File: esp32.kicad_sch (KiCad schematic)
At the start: 39 parts, among them U5 ESP32-S3R8, U6 W25Q128JVSIQ, Y1 40MHz

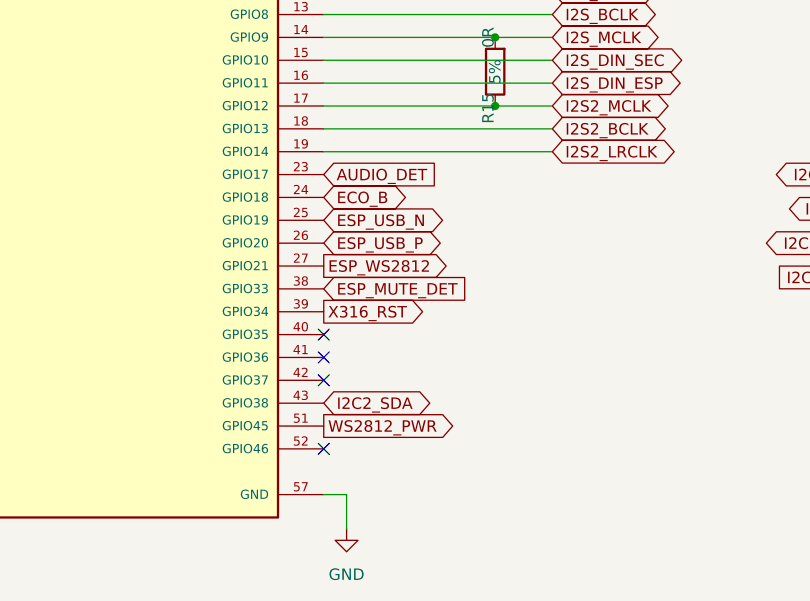
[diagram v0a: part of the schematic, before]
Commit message: rev2 update
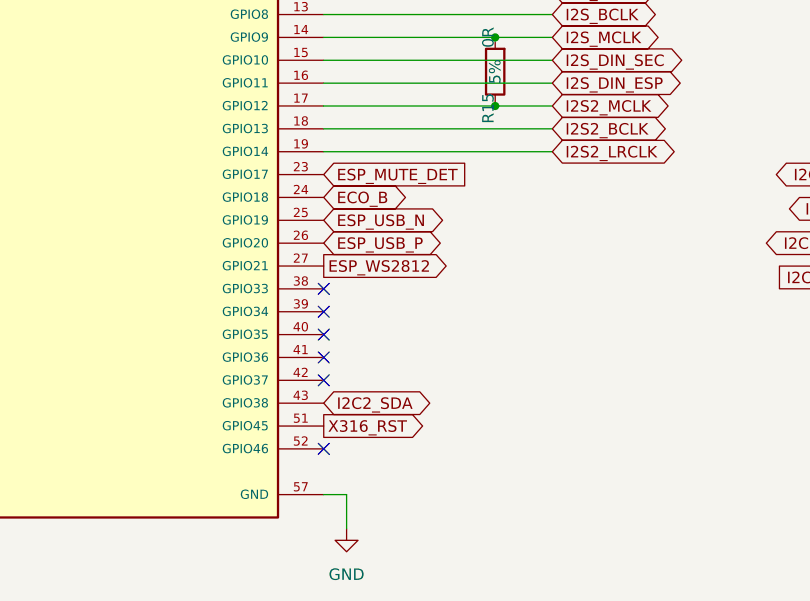
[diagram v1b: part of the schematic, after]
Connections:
- net AUDIO_DET is gone; now on net ESP_MUTE_DET: U5.23 (GPIO17)
- net WS2812_PWR is gone; now on net X316_RST: U5.51 (GPIO45)
- net ESP_MUTE_DET: no longer U5.38 (GPIO33)
- net X316_RST: no longer U5.39 (GPIO34)
- no-connect marks 6 -> 8
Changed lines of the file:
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@@
+	)
+	(no_connect
+		(at 162.56 116.84)
 	)
 	(no_connect
 		(at 162.56 134.62)
+	)
+	(no_connect
+		(at 162.56 119.38)
 	)
 	(no_connect
@@
 		)
 	)
+	(global_label "ESP_MUTE_DET"
+		(shape input)
+		(at 162.56 104.14 0)
+		(fields_autoplaced yes)
+		(effects
+			(font
+				(size 1.27 1.27)
+			)
+			(justify left)
+		)
+		(property "Intersheetrefs" "${INTERSHEET_REFS}"
+			(at 179.394 104.14 0)
+			(effects
+				(font
+					(size 1.27 1.27)
+				)
+				(justify left)
+				(hide yes)
+			)
+		)
+	)
 	(global_label "ESP_RX0"
 		(shape input)
@@
 		)
 	)
-	(global_label "X316_RST"
-		(shape output)
-		(at 162.56 119.38 0)
-		(fields_autoplaced yes)
-		(effects
-			(font
-				(size 1.27 1.27)
-			)
-			(justify left)
-		)
-		(property "Intersheetrefs" "${INTERSHEET_REFS}"
-			(at 174.7979 119.38 0)
-			(effects
-				(font
-					(size 1.27 1.27)
-				)
-				(justify left)
-				(hide yes)
-			)
-		)
-	)
 	(global_label "I2C_SCL"
 		(shape output)
@@
 		)
 	)
-	(global_label "ESP_MUTE_DET"
-		(shape input)
-		(at 162.56 116.84 0)
-		(fields_autoplaced yes)
-		(effects
-			(font
-				(size 1.27 1.27)
-			)
-			(justify left)
-		)
-		(property "Intersheetrefs" "${INTERSHEET_REFS}"
-			(at 179.394 116.84 0)
-			(effects
-				(font
-					(size 1.27 1.27)
-				)
-				(justify left)
-				(hide yes)
-			)
-		)
-	)
 	(global_label "ECO_B"
 		(shape bidirectional)
@@
 		)
 	)
+	(global_label "X316_RST"
+		(shape output)
+		(at 162.56 132.08 0)
+		(fields_autoplaced yes)
+		(effects
+			(font
+				(size 1.27 1.27)
+			)
+			(justify left)
+		)
+		(property "Intersheetrefs" "${INTERSHEET_REFS}"
+			(at 174.7979 132.08 0)
+			(effects
+				(font
+					(size 1.27 1.27)
+				)
+				(justify left)
+				(hide yes)
+			)
+		)
+	)
 	(global_label "I2S2_LRCLK"
 		(shape bidirectional)
@@
 		)
 	)
-	(global_label "WS2812_PWR"
-		(shape output)
-		(at 162.56 132.08 0)
-		(fields_autoplaced yes)
-		(effects
-			(font
-				(size 1.27 1.27)
-			)
-			(justify left)
-		)
-		(property "Intersheetrefs" "${INTERSHEET_REFS}"
-			(at 178.0031 132.08 0)
-			(effects
-				(font
-					(size 1.27 1.27)
-				)
-				(justify left)
-				(hide yes)
-			)
-		)
-	)
 	(global_label "I2S_LRCK"
 		(shape bidirectional)
@@
 			(effects
 				(font
-					(size 1.27 1.27)
-				)
-				(justify left)
-				(hide yes)
-			)
-		)
-	)
-	(global_label "AUDIO_DET"
-		(shape input)
-		(at 162.56 104.14 0)
-		(fields_autoplaced yes)
-		(effects
-			(font
-				(size 1.27 1.27)
-			)
-			(justify left)
-		)
-		(property "Intersheetrefs" "${INTERSHEET_REFS}"
-			(at 175.5238 104.14 0)
-			(effects
-				(font
